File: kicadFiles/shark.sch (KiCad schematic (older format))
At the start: 260 parts, among them J1 USB_C_Receptacle, J2 Conn_01x04_Male, Q1 AO4406AL, SW1 MXSwitch, SW10 MXSwitch, SW11 MXSwitch, SW12 MXSwitch, SW13 MXSwitch, SW14 MXSwitch, SW15 MXSwitch, SW16 MXSwitch, SW17 MXSwitch, SW18 MXSwitch, SW19 MXSwitch, SW2 MXSwitch, SW20 MXSwitch, SW21 MXSwitch, SW22 MXSwitch, SW23 MXSwitch, SW24 MXSwitch, SW25 MXSwitch, SW26 MXSwitch, SW27 MXSwitch, SW28 MXSwitch, SW29 MXSwitch, SW3 MXSwitch, SW30 MXSwitch, SW31 MXSwitch, SW32 MXSwitch, SW33 MXSwitch, SW34 MXSwitch, SW35 MXSwitch, SW36 MXSwitch, SW37 MXSwitch, SW38 MXSwitch, SW39 MXSwitch, SW4 MXSwitch, SW40 MXSwitch, SW41 MXSwitch, SW42 MXSwitch, SW43 MXSwitch, SW44 MXSwitch, SW45 MXSwitch, SW46 MXSwitch, SW47 MXSwitch, SW48 MXSwitch, SW49 MXSwitch, SW5 MXSwitch, SW50 MXSwitch, SW51 MXSwitch, SW6 MXSwitch, SW7 MXSwitch, SW8 MXSwitch, SW9 MXSwitch, U1 STM32F303CCT6, U2 MCP1700-3302E_SOT23, Y1 8MHz

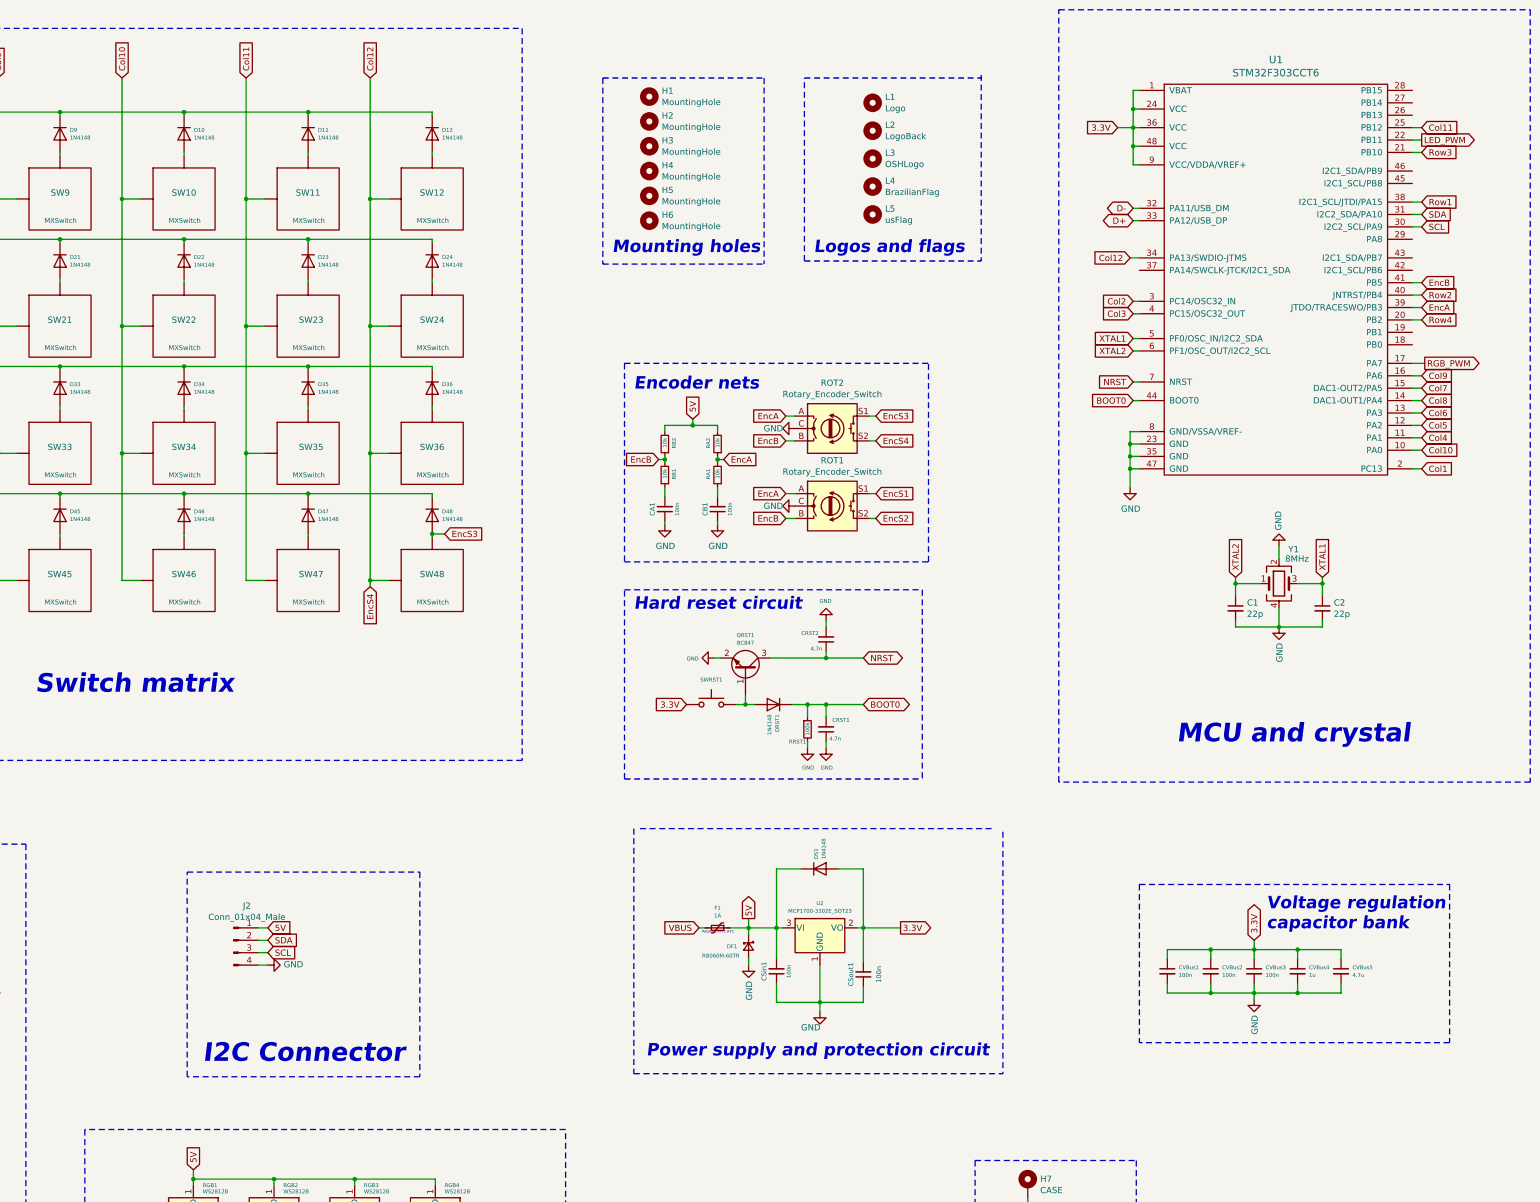
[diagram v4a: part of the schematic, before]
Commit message: [Feature] Added header pins for the extra MCU pins
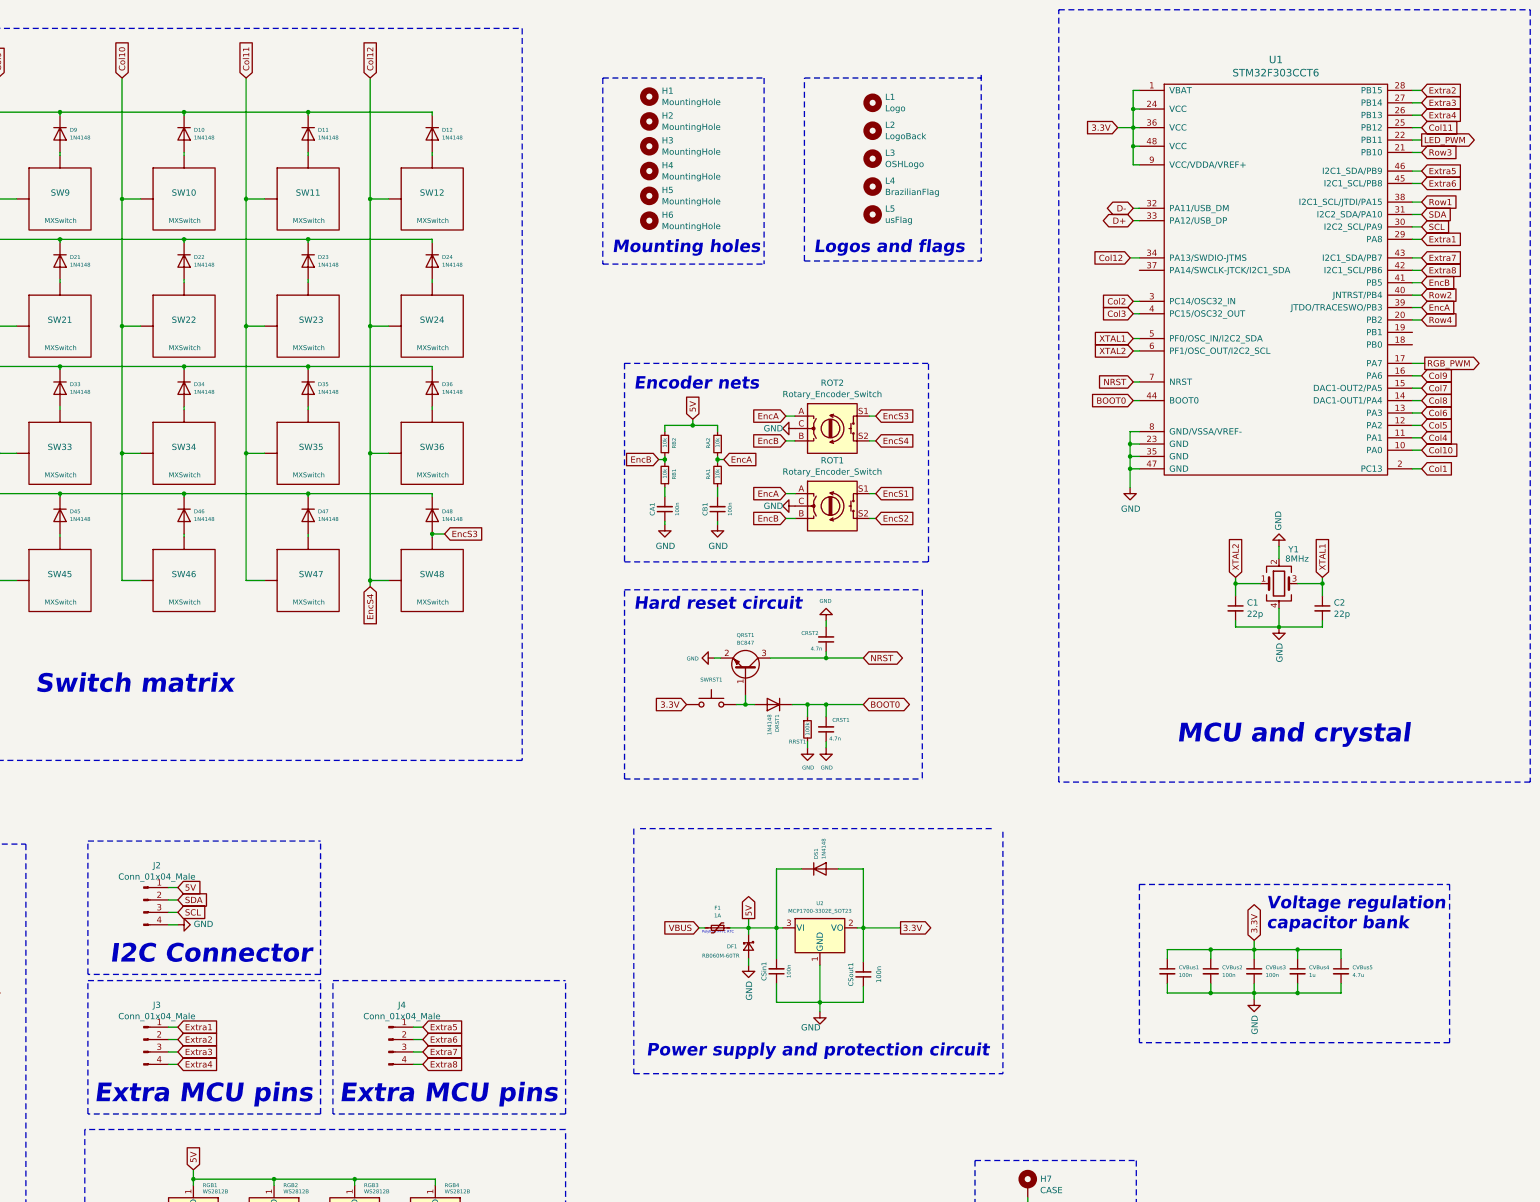
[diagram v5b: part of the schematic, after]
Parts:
- added J3, J4: Conn_01x04_Male, acheronConnectors:4pinHeader, symbol Connector:Conn_01x04_Male
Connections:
- net Extra4: now reaches U1.26 (PB13)
- net Extra4: now also J3.4 (Pin_4)
- net Extra3: now reaches U1.27 (PB14)
- net Extra3: now also J3.3 (Pin_3)
- net Extra2: now reaches U1.28 (PB15)
- net Extra2: now also J3.2 (Pin_2)
- net Extra1: now reaches U1.29 (PA8)
- net Extra1: now also J3.1 (Pin_1)
- net Extra8: now reaches U1.42 (I2C1_SCL/PB6)
- net Extra8: now also J4.4 (Pin_4)
- net Extra7: now reaches U1.43 (I2C1_SDA/PB7)
- net Extra7: now also J4.3 (Pin_3)
- net Extra6: now reaches U1.45 (I2C1_SCL/PB8)
- net Extra6: now also J4.2 (Pin_2)
- net Extra5: now reaches U1.46 (I2C1_SDA/PB9)
- net Extra5: now also J4.1 (Pin_1)
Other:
- note added: "Extra MCU pins"
- moved on the sheet: J2
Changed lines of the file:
@@
 Title "SharkPCB"
 Date "2019-03-13"
-Rev "Rev 3.1.3"
+Rev "Rev 3.1.4"
 Comp "Gondolin Electronics"
 Comment1 ""
@@
 L Connector:Conn_01x04_Male J2
 U 1 1 5C8FE384
-P 11875 9950
-F 0 "J2" H 11981 10228 50  0000 C CNN
-F 1 "Conn_01x04_Male" H 11981 10137 50  0000 C CNN
-F 2 "acheronConnectors:4pinHeader" H 11875 9950 50  0001 C CNN
-F 3 "~" H 11875 9950 50  0001 C CNN
-	1    11875 9950
+P 11150 9625
+F 0 "J2" H 11256 9903 50  0000 C CNN
+F 1 "Conn_01x04_Male" H 11256 9812 50  0000 C CNN
+F 2 "acheronConnectors:4pinHeader" H 11150 9625 50  0001 C CNN
+F 3 "~" H 11150 9625 50  0001 C CNN
+	1    11150 9625
 	1    0    0    -1
 $EndComp
 Wire Wire Line
-	12075 9850 12150 9850
-Text GLabel 12150 9850 2    50   Input ~ 0
+	11350 9525 11425 9525
+Text GLabel 11425 9525 2    50   Input ~ 0
 5V
 Wire Wire Line
-	12075 10150 12150 10150
+	11350 9825 11425 9825
 $Comp
 L power:GND #PWR0102
 U 1 1 5C9D3CEB
-P 12150 10150
-F 0 "#PWR0102" H 12150 9900 50  0001 C CNN
-F 1 "GND" V 12155 10022 50  0000 R CNN
-F 2 "" H 12150 10150 50  0001 C CNN
-F 3 "" H 12150 10150 50  0001 C CNN
-	1    12150 10150
+P 11425 9825
+F 0 "#PWR0102" H 11425 9575 50  0001 C CNN
+F 1 "GND" V 11430 9697 50  0000 R CNN
+F 2 "" H 11425 9825 50  0001 C CNN
+F 3 "" H 11425 9825 50  0001 C CNN
+	1    11425 9825
 	0    -1   -1   0
 $EndComp
 Wire Wire Line
-	12075 9950 12150 9950
-Text GLabel 12150 9950 2    50   Input ~ 0
+	11350 9625 11425 9625
+Text GLabel 11425 9625 2    50   Input ~ 0
 SDA
-Text GLabel 12150 10050 2    50   Input ~ 0
+Text GLabel 11425 9725 2    50   Input ~ 0
 SCL
 Wire Wire Line
-	12150 10050 12075 10050
+	11425 9725 11350 9725
 Wire Notes Line width 20
-	11500 9400 13375 9400
+	10700 9150 12575 9150
 Wire Notes Line width 20
-	13375 9400 13375 11050
-Wire Notes Line width 20
-	13375 11050 11500 11050
-Wire Notes Line width 20
-	11500 11050 11500 9400
-Text Notes 11625 10950 0    150  Italic 30
+	12575 10225 10700 10225
+Text Notes 10875 10150 0    150  Italic 30
 I2C Connector
 Text GLabel 21450 4200 2    50   Input ~ 0
@@
 Wire Wire Line
 	19100 4450 19175 4450
+Text GLabel 21450 4300 2    50   Input ~ 0
+Extra1
+Text GLabel 21450 3100 2    50   Input ~ 0
+Extra2
+Text GLabel 21450 3200 2    50   Input ~ 0
+Extra3
+Text GLabel 21450 3300 2    50   Input ~ 0
+Extra4
+Wire Wire Line
+	21375 3300 21450 3300
+Wire Wire Line
+	21450 3200 21375 3200
+Wire Wire Line
+	21375 3100 21450 3100
+Wire Wire Line
+	21450 4300 21375 4300
+Wire Notes Line width 20
+	12575 10225 12575 9150
+Wire Notes Line width 20
+	10700 10225 10700 9150
+$Comp
+L Connector:Conn_01x04_Male J3
+U 1 1 5D18EBC8
+P 11150 10750
+F 0 "J3" H 11256 11028 50  0000 C CNN
+F 1 "Conn_01x04_Male" H 11256 10937 50  0000 C CNN
+F 2 "acheronConnectors:4pinHeader" H 11150 10750 50  0001 C CNN
+F 3 "~" H 11150 10750 50  0001 C CNN
+	1    11150 10750
+	1    0    0    -1
+$EndComp
+Wire Wire Line
+	11350 10650 11425 10650
+Text GLabel 11425 10650 2    50   Input ~ 0
+Extra1
+Wire Wire Line
+	11350 10950 11425 10950
+Wire Wire Line
+	11350 10750 11425 10750
+Text GLabel 11425 10750 2    50   Input ~ 0
+Extra2
+Text GLabel 11425 10850 2    50   Input ~ 0
+Extra3
+Wire Wire Line
+	11425 10850 11350 10850
+Wire Notes Line width 20
+	10700 10275 12575 10275
+Wire Notes Line width 20
+	12575 11350 10700 11350
+Text Notes 10750 11275 0    150  Italic 30
+Extra MCU pins
+Wire Notes Line width 20
+	12575 11350 12575 10275
+Wire Notes Line width 20
+	10700 11350 10700 10275
+Text GLabel 11425 10950 2    50   Input ~ 0
+Extra4
+Text GLabel 21450 3750 2    50   Input ~ 0
+Extra5
+Text GLabel 21450 3850 2    50   Input ~ 0
+Extra6
+Text GLabel 21450 4450 2    50   Input ~ 0
+Extra7
+Text GLabel 21450 4550 2    50   Input ~ 0
+Extra8
+Wire Wire Line
+	21450 4550 21375 4550
+Wire Wire Line
+	21375 4450 21450 4450
+Wire Wire Line
+	21450 3750 21375 3750
+Wire Wire Line
+	21375 3850 21450 3850
+$Comp
+L Connector:Conn_01x04_Male J4
+U 1 1 5D3B4464
+P 13125 10750
+F 0 "J4" H 13231 11028 50  0000 C CNN
+F 1 "Conn_01x04_Male" H 13231 10937 50  0000 C CNN
+F 2 "acheronConnectors:4pinHeader" H 13125 10750 50  0001 C CNN
+F 3 "~" H 13125 10750 50  0001 C CNN
+	1    13125 10750
+	1    0    0    -1
+$EndComp
+Wire Wire Line
+	13325 10650 13400 10650
+Text GLabel 13400 10650 2    50   Input ~ 0
+Extra5
+Wire Wire Line
+	13325 10950 13400 10950
+Wire Wire Line
+	13325 10750 13400 10750
+Text GLabel 13400 10750 2    50   Input ~ 0
+Extra6
+Text GLabel 13400 10850 2    50   Input ~ 0
+Extra7
+Wire Wire Line
+	13400 10850 13325 10850
+Wire Notes Line width 20
+	12675 10275 14550 10275
+Wire Notes Line width 20
+	14550 11350 12675 11350
+Text Notes 12725 11275 0    150  Italic 30
+Extra MCU pins
+Wire Notes Line width 20
+	14550 11350 14550 10275
+Wire Notes Line width 20
+	12675 11350 12675 10275
+Text GLabel 13400 10950 2    50   Input ~ 0
+Extra8
 $EndSCHEMATC

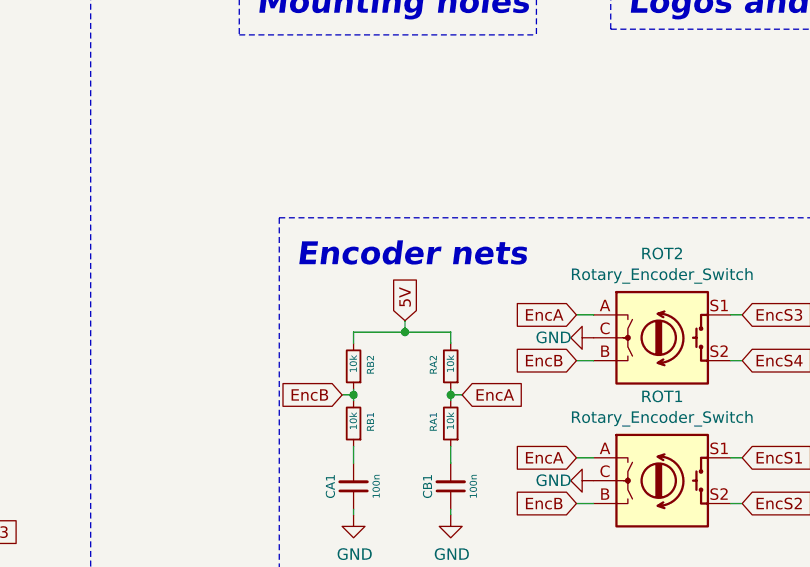
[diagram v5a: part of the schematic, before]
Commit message: [Fix] Used 3.3V for encoder VCC instead of 5V
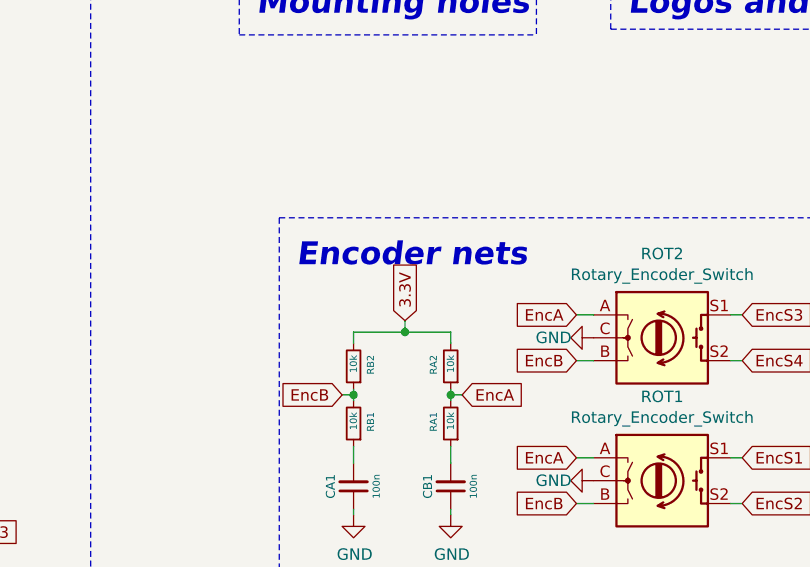
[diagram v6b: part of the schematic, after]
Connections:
- net 3.3V: now also RA2.2, RB2.2
- net 5V: no longer RA2.2, RB2.2
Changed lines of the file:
@@
 Title "SharkPCB"
 Date "2019-03-13"
-Rev "Rev 3.1.4"
+Rev "Rev 3.1.5"
 Comp "Gondolin Electronics"
 Comment1 ""
@@
 EncA
 Text GLabel 15575 5750 1    50   Input ~ 0
-5V
+3.3V
 Wire Wire Line
 	15300 6075 15350 6075

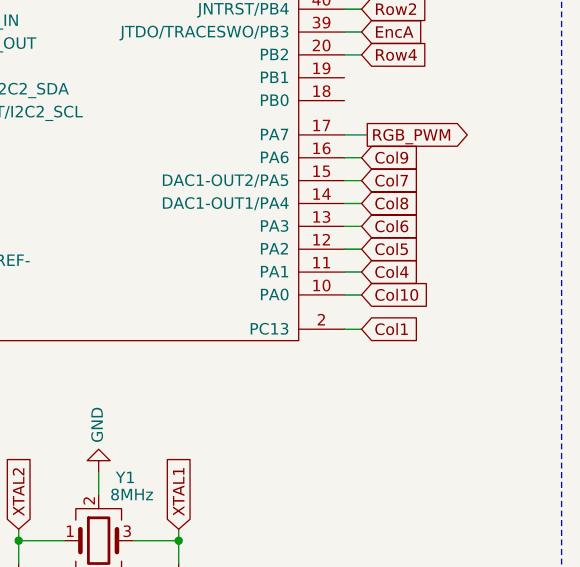
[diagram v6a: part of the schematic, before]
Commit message: [Maintenance] Moved some SMD parts to the bottom layer to ensure no problems with switch mounting
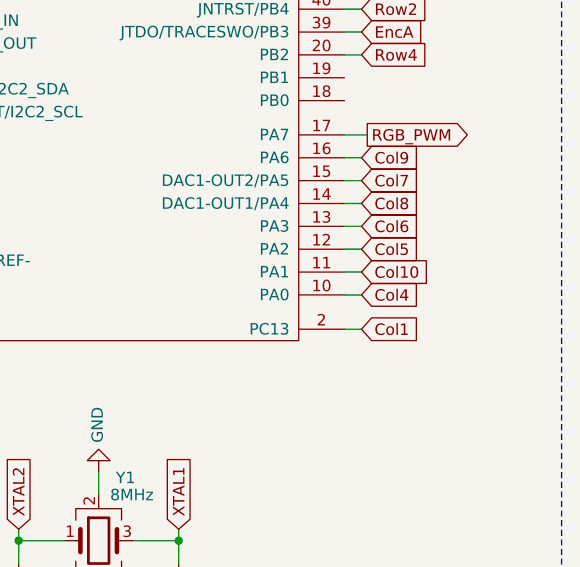
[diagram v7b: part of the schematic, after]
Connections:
- net Col10: now also U1.11 (PA1); no longer U1.10 (PA0)
- net Col4: now also U1.10 (PA0); no longer U1.11 (PA1)
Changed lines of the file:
@@
 Wire Wire Line
 	21450 3400 21375 3400
-Text GLabel 21450 6000 2    50   Input ~ 0
+Text GLabel 21450 5900 2    50   Input ~ 0
 Col10
 Wire Wire Line
-	21450 6000 21375 6000
+	21450 5900 21375 5900
 $Comp
 L Mechanical:MountingHole L2
@@
 Wire Wire Line
 	19125 4900 19175 4900
-Text GLabel 21450 5900 2    50   Input ~ 0
+Text GLabel 21450 6000 2    50   Input ~ 0
 Col4
 Wire Wire Line
-	21450 5900 21375 5900
+	21450 6000 21375 6000
 Text GLabel 21450 5800 2    50   Input ~ 0
 Col5

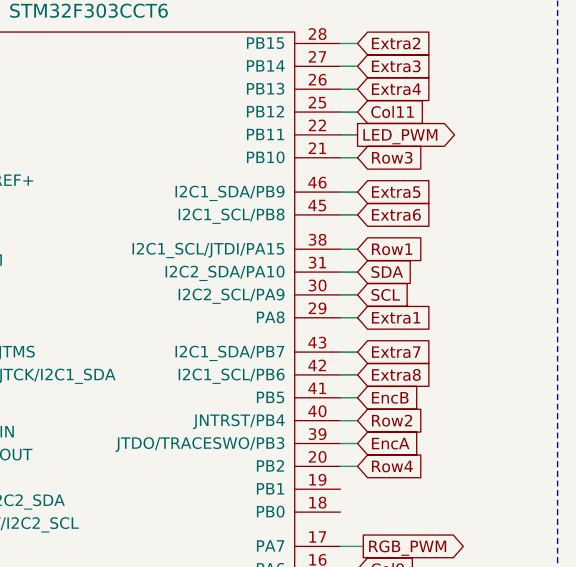
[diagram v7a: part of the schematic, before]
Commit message: [Fix] Removed inconsistencies in BOM and added correct gerber
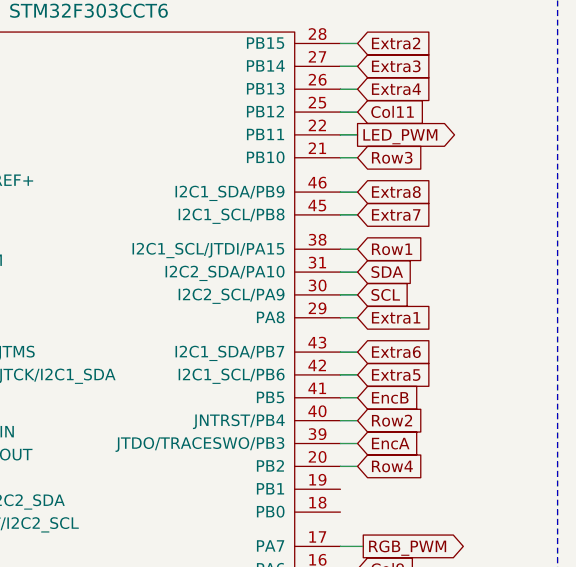
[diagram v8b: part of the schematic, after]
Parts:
- CVBus4: footprint Capacitor_SMD:C_0402_1005Metric -> Capacitor_SMD:C_0805_2012Metric_Pad1.15x1.40mm_HandSolder
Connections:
- net Extra5: now also U1.42 (I2C1_SCL/PB6); no longer U1.46 (I2C1_SDA/PB9)
- net Extra6: now also U1.43 (I2C1_SDA/PB7); no longer U1.45 (I2C1_SCL/PB8)
- net Extra7: now also U1.45 (I2C1_SCL/PB8); no longer U1.43 (I2C1_SDA/PB7)
- net Extra8: now also U1.46 (I2C1_SDA/PB9); no longer U1.42 (I2C1_SCL/PB6)
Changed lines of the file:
@@
 Sheet 1 1
 Title "SharkPCB"
-Date "2019-03-13"
-Rev "Rev 3.1.5"
+Date "2019-03-20"
+Rev "3.1.6"
 Comp "Gondolin Electronics"
 Comment1 ""
@@
 F 0 "CVBus4" H 20542 10231 31  0000 L CNN
 F 1 "1u" H 20542 10169 31  0000 L CNN
-F 2 "Capacitor_SMD:C_0402_1005Metric" H 20450 10200 50  0001 C CNN
+F 2 "Capacitor_SMD:C_0805_2012Metric_Pad1.15x1.40mm_HandSolder" H 20450 10200 50  0001 C CNN
 F 3 "~" H 20450 10200 50  0001 C CNN
 	1    20450 10200
@@
 Extra4
 Text GLabel 21450 3750 2    50   Input ~ 0
-Extra5
+Extra8
 Text GLabel 21450 3850 2    50   Input ~ 0
-Extra6
-Text GLabel 21450 4450 2    50   Input ~ 0
 Extra7
+Text GLabel 21450 4450 2    50   Input ~ 0
+Extra6
 Text GLabel 21450 4550 2    50   Input ~ 0
-Extra8
+Extra5
 Wire Wire Line
 	21450 4550 21375 4550
